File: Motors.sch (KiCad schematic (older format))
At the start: 17 parts, among them J2 LEFT_MOTOR, J3 RIGHT_MOTOR, U3 VNH5019, U4 VNH5019

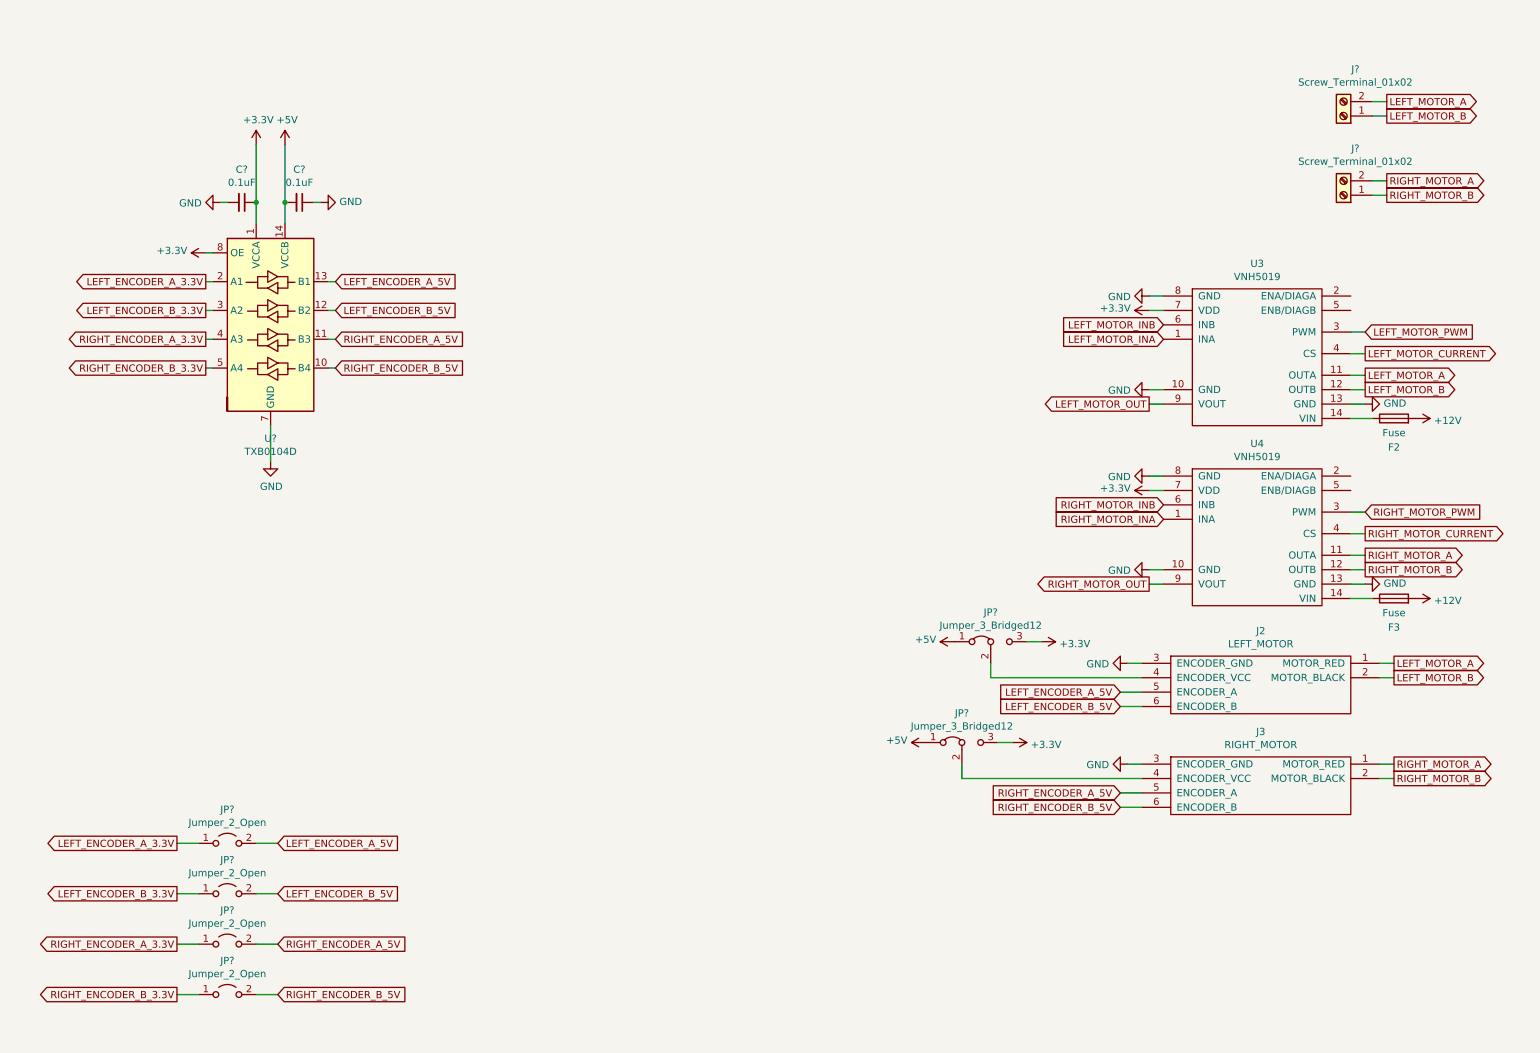
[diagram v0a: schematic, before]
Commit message: Most of rev B
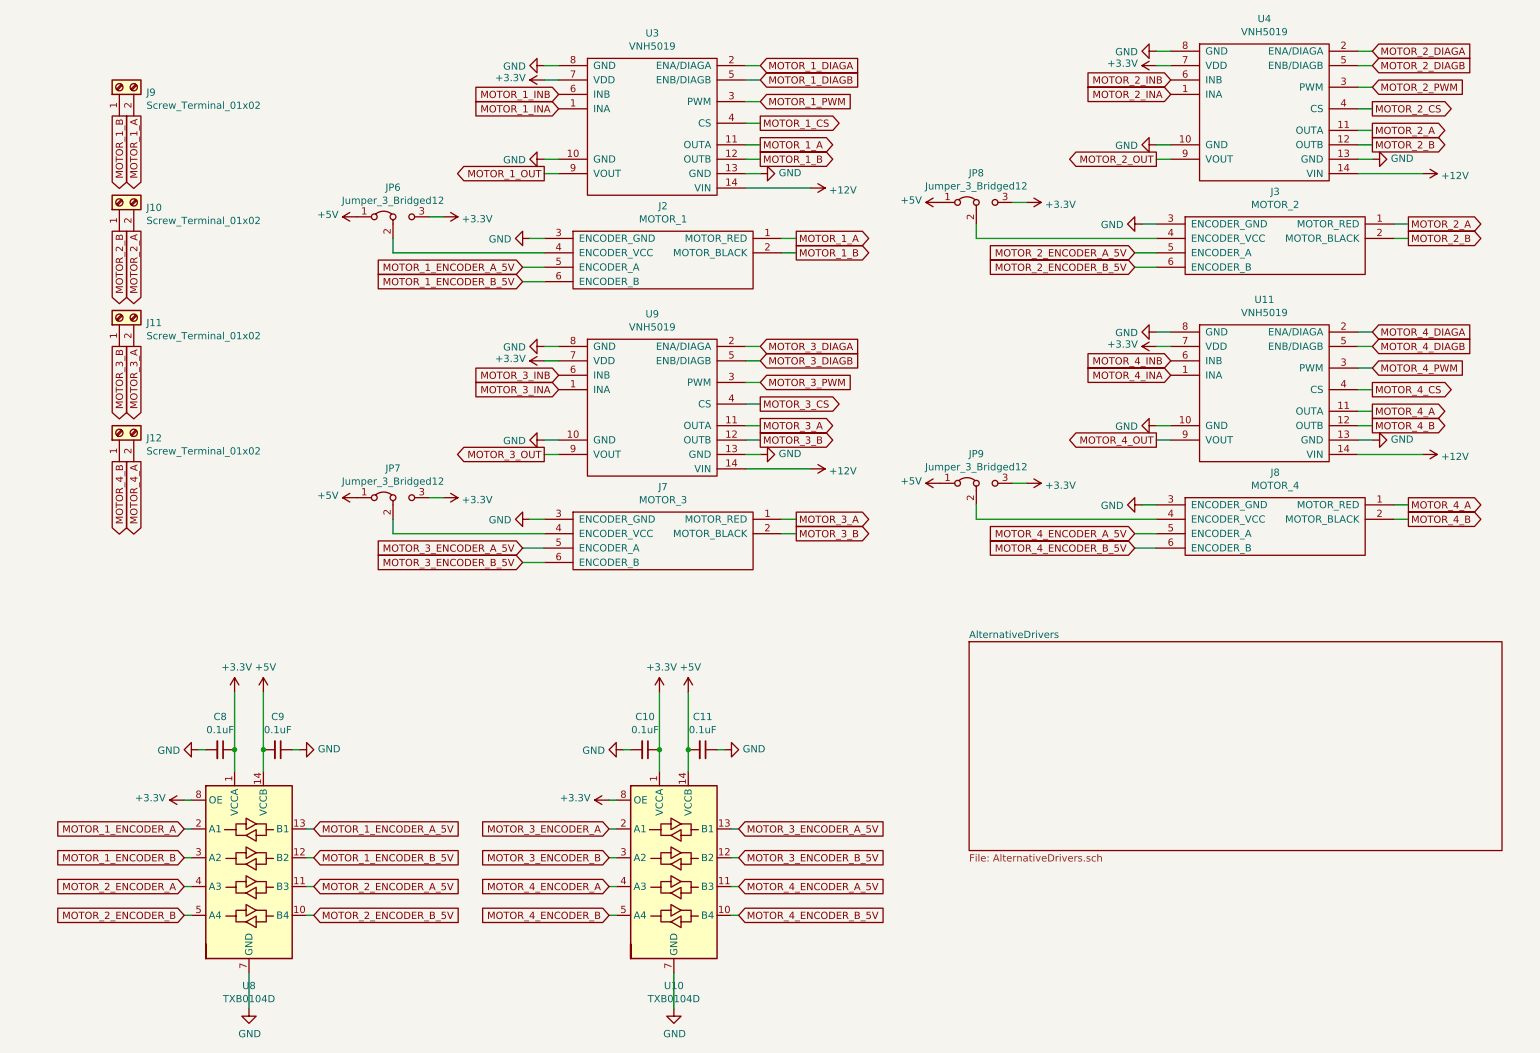
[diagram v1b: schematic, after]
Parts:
- removed F2, F3: Fuse, Fuse:Fuse_0805_2012Metric_Pad1.15x1.40mm_HandSolder, symbol Device:Fuse
- removed J? (x2): Screw_Terminal_01x02, symbol Connector:Screw_Terminal_01x02
- removed JP? (x4): Jumper_2_Open, symbol Jumper:Jumper_2_Open
- added C10, C11: 0.1uF, Capacitor_SMD:C_0603_1608Metric_Pad1.05x0.95mm_HandSolder, symbol Device:C_Small
- added J10, J11, J12, J9: Screw_Terminal_01x02, TerminalBlock_Phoenix:TerminalBlock_Phoenix_MKDS-3-2-5.08_1x02_P5.08mm_Horizontal, symbol Connector:Screw_Terminal_01x02
- added J7: MOTOR_3, Connector_PinHeader_2.54mm:PinHeader_1x06_P2.54mm_Vertical, symbol pololu_parts:MOTOR_CONNECTOR
- added J8: MOTOR_4, Connector_PinHeader_2.54mm:PinHeader_1x06_P2.54mm_Vertical, symbol pololu_parts:MOTOR_CONNECTOR
- added JP7, JP9: Jumper_3_Bridged12, Jumper:SolderJumper-3_P1.3mm_Bridged12_RoundedPad1.0x1.5mm, symbol Jumper:Jumper_3_Bridged12
- added U10: TXB0104D, Package_SO:SOIC-14_3.9x8.7mm_P1.27mm, symbol Logic_LevelTranslator:TXB0104D
- added U11, U9: VNH5019, TurtlebotController:Pololu_VNH5019_Carrier, symbol pololu_parts:VNH5019
- C8, C9: renamed from C?; footprint (none) -> Capacitor_SMD:C_0603_1608Metric_Pad1.05x0.95mm_HandSolder
- J2: value LEFT_MOTOR -> MOTOR_1
- J3: value RIGHT_MOTOR -> MOTOR_2
- JP6, JP8: renamed from JP?; footprint (none) -> Jumper:SolderJumper-3_P1.3mm_Bridged12_RoundedPad1.0x1.5mm
- gave numbers to parts that had none: 1
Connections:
- net +12V: now also U3.14 (VIN), U4.14 (VIN), U11.14 (VIN), U9.14 (VIN)
- net +3V3: now also C10.1, JP7.3 (B), JP9.3 (B), U10.1 (VCCA), U10.8 (OE), U11.7 (VDD), U9.7 (VDD)
- net +5V: now also C11.2, JP7.1 (A), JP9.1 (A), U10.14 (VCCB)
- net GND: now also C10.2, C11.1, J7.3 (ENCODER_GND), J8.3 (ENCODER_GND), U10.7 (GND), U11.10 (GND), U11.13 (GND), U11.8 (GND), U9.10 (GND), U9.13 (GND), U9.8 (GND)
- net MOTOR_1_DIAGA: now reaches U3.2 (ENA/DIAGA)
- net MOTOR_1_DIAGB: now reaches U3.5 (ENB/DIAGB)
- net MOTOR_2_DIAGA: now reaches U4.2 (ENA/DIAGA)
- net MOTOR_2_DIAGB: now reaches U4.5 (ENB/DIAGB)
- net LEFT_ENCODER_A_3.3V renamed MOTOR_1_ENCODER_A
- net LEFT_ENCODER_A_5V renamed MOTOR_1_ENCODER_A_5V
- net LEFT_ENCODER_B_3.3V renamed MOTOR_1_ENCODER_B
- net LEFT_ENCODER_B_5V renamed MOTOR_1_ENCODER_B_5V
- net LEFT_MOTOR_A renamed MOTOR_1_A
- net MOTOR_1_A: now also J9.2 (Pin_2)
- net LEFT_MOTOR_B renamed MOTOR_1_B
- net MOTOR_1_B: now also J9.1 (Pin_1)
- net LEFT_MOTOR_CURRENT renamed MOTOR_1_CS
- net LEFT_MOTOR_INA renamed MOTOR_1_INA
- net LEFT_MOTOR_INB renamed MOTOR_1_INB
- net LEFT_MOTOR_OUT renamed MOTOR_1_OUT
- net LEFT_MOTOR_PWM renamed MOTOR_1_PWM
- net RIGHT_ENCODER_A_3.3V renamed MOTOR_2_ENCODER_A
- net RIGHT_ENCODER_A_5V renamed MOTOR_2_ENCODER_A_5V
- net RIGHT_ENCODER_B_3.3V renamed MOTOR_2_ENCODER_B
- net RIGHT_ENCODER_B_5V renamed MOTOR_2_ENCODER_B_5V
- net RIGHT_MOTOR_A renamed MOTOR_2_A
- net MOTOR_2_A: now also J10.2 (Pin_2)
- net RIGHT_MOTOR_B renamed MOTOR_2_B
- net MOTOR_2_B: now also J10.1 (Pin_1)
- net RIGHT_MOTOR_CURRENT renamed MOTOR_2_CS
- net RIGHT_MOTOR_INA renamed MOTOR_2_INA
- net RIGHT_MOTOR_INB renamed MOTOR_2_INB
- net RIGHT_MOTOR_OUT renamed MOTOR_2_OUT
- net RIGHT_MOTOR_PWM renamed MOTOR_2_PWM
- new net: J7.4 (ENCODER_VCC), JP7.2 (C)
- new net: J8.4 (ENCODER_VCC), JP9.2 (C)
- new net MOTOR_3_A: J11.2 (Pin_2), J7.1 (MOTOR_RED), U9.11 (OUTA)
- new net MOTOR_3_B: J11.1 (Pin_1), J7.2 (MOTOR_BLACK), U9.12 (OUTB)
- new net MOTOR_3_CS: U9.4 (CS)
- new net MOTOR_3_DIAGA: U9.2 (ENA/DIAGA)
- new net MOTOR_3_DIAGB: U9.5 (ENB/DIAGB)
- new net MOTOR_3_ENCODER_A: U10.2 (A1)
- new net MOTOR_3_ENCODER_A_5V: J7.5 (ENCODER_A), U10.13 (B1)
- new net MOTOR_3_ENCODER_B: U10.3 (A2)
- new net MOTOR_3_ENCODER_B_5V: J7.6 (ENCODER_B), U10.12 (B2)
- new net MOTOR_3_INA: U9.1 (INA)
- new net MOTOR_3_INB: U9.6 (INB)
- new net MOTOR_3_OUT: U9.9 (VOUT)
- new net MOTOR_3_PWM: U9.3 (PWM)
- new net MOTOR_4_A: J12.2 (Pin_2), J8.1 (MOTOR_RED), U11.11 (OUTA)
- new net MOTOR_4_B: J12.1 (Pin_1), J8.2 (MOTOR_BLACK), U11.12 (OUTB)
- new net MOTOR_4_CS: U11.4 (CS)
- new net MOTOR_4_DIAGA: U11.2 (ENA/DIAGA)
- new net MOTOR_4_DIAGB: U11.5 (ENB/DIAGB)
- new net MOTOR_4_ENCODER_A: U10.4 (A3)
- new net MOTOR_4_ENCODER_A_5V: J8.5 (ENCODER_A), U10.11 (B3)
- new net MOTOR_4_ENCODER_B: U10.5 (A4)
- new net MOTOR_4_ENCODER_B_5V: J8.6 (ENCODER_B), U10.10 (B4)
- new net MOTOR_4_INA: U11.1 (INA)
- new net MOTOR_4_INB: U11.6 (INB)
- new net MOTOR_4_OUT: U11.9 (VOUT)
- new net MOTOR_4_PWM: U11.3 (PWM)
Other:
- moved on the sheet: C8, C9, J2, J3, JP6, JP8, U3, U4, U8
